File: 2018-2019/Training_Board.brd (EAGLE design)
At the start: 65 x 30 mm, 14 parts, among them IC1 ATMEGA328-20P, X1 JST-PH2

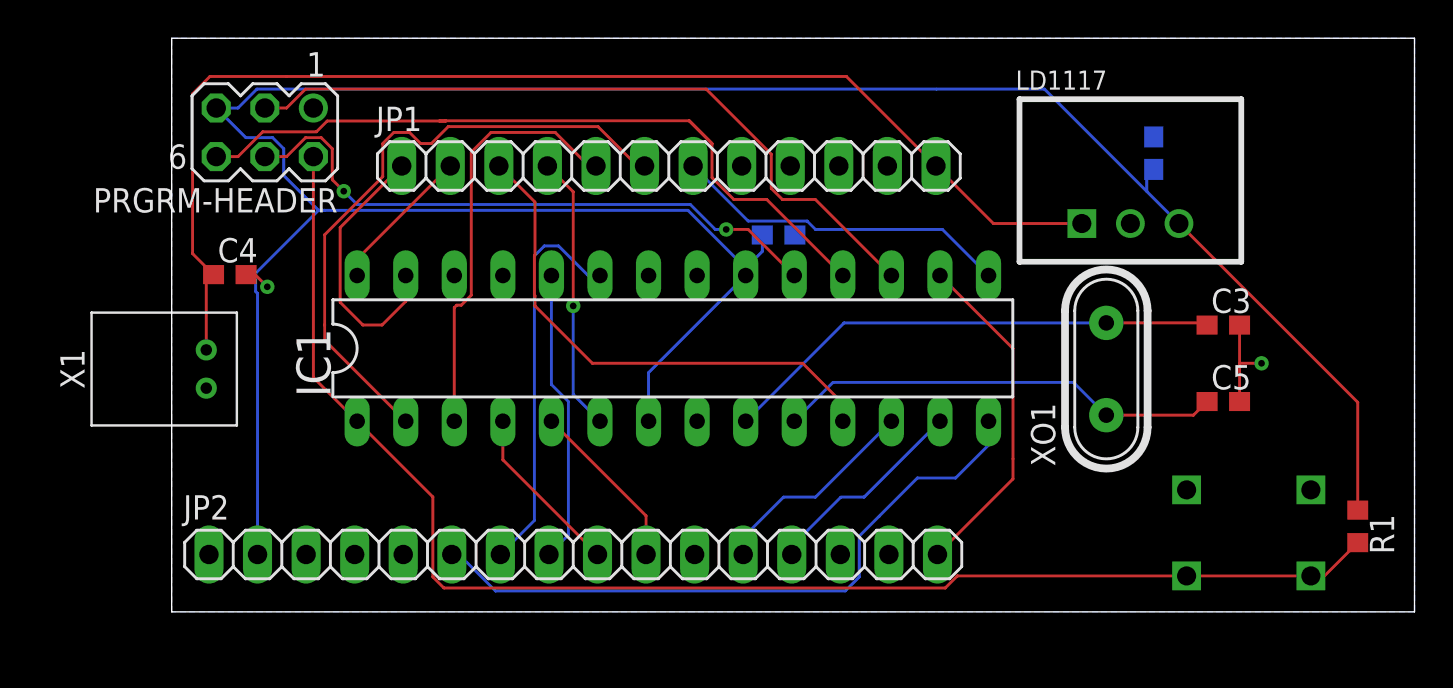
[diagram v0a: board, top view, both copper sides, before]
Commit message: Routed with larger trace widths and corrected pinouts
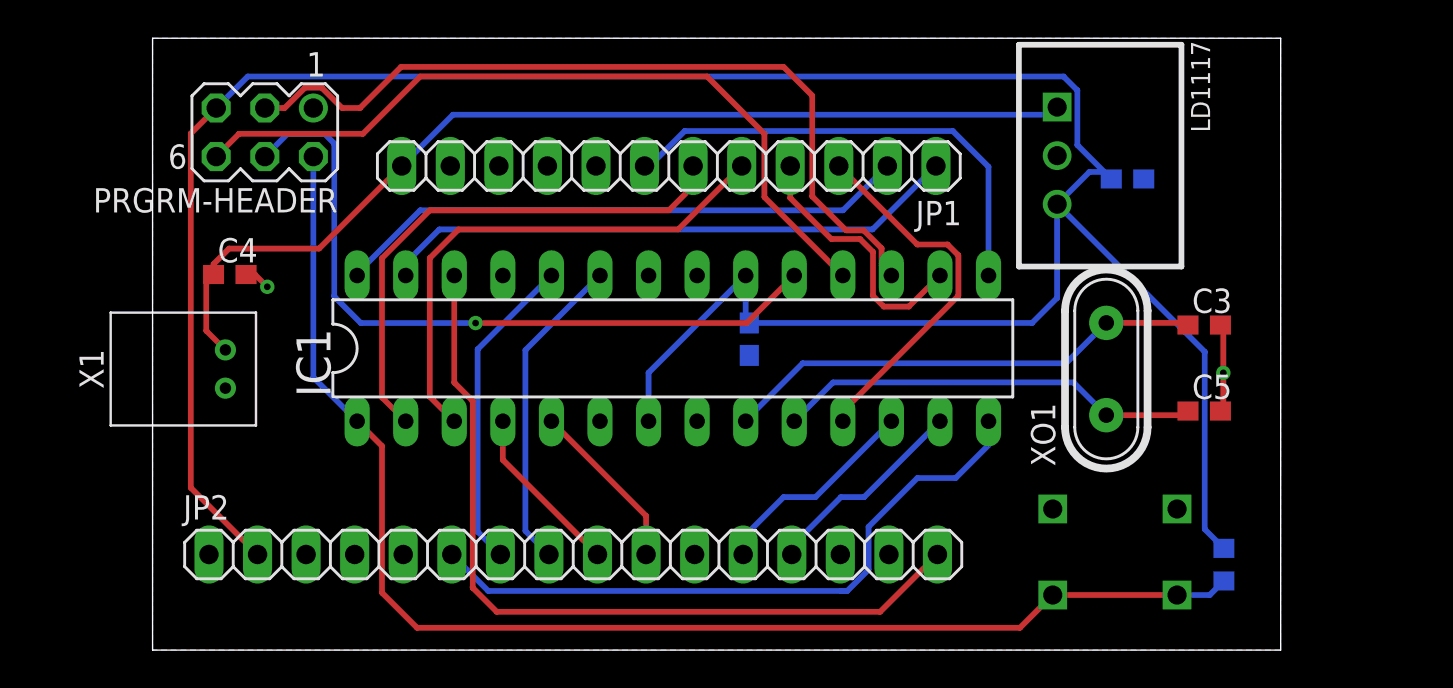
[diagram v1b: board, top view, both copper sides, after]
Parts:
- moved R1 7.28 mm to (55.0, 2.47), flipped to the bottom
- moved S1 7.07 mm to (46.1, 0.88)
- moved C1 5.66 mm to (30.2, 14.3), turned to 270 degrees
- moved LD1117 5.22 mm to (46.3, 23.9), turned to 270 degrees
- moved C2 1.92 mm to (50.0, 22.6), turned to 180 degrees
- moved C5 1.12 mm to (54.0, 10.5)
- moved C3 1.00 mm to (54.0, 15.0)
- moved X1 1.00 mm to (2.81, 12.7)
- turned JP1 to 180 degrees
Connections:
- net LIFT_A: now also IC1.16; no longer IC1.6
- net LINE_OUT_1: now also IC1.24; no longer IC1.23
- net LINE_OUT_2: now also IC1.23; no longer IC1.24
- net MOTOR_FAULT: now also IC1.26; no longer IC1.16
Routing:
- net MOTOR_FAULT: track 17.8 -> 42.8 mm
- net SCL: track 7.75 -> 30.2 mm
- net SDA: track 14.2 -> 30.5 mm
- net VBAT: track 64.1 -> 52.6 mm
- net LIFT_B: track 27.3 -> 19.4 mm
- net LEFT_B: track 17.8 -> 25.2 mm
- net SCK: track 32.0 -> 38.0 mm, vias 2 -> 1
- net RIGHT_B: track 22.3 -> 27.4 mm
- net RIGHT_A: track 32.9 -> 27.9 mm
- net MOSI: track 38.3 -> 42.7 mm
- net RST: track 74.2 -> 70.1 mm
- net LINE_OUT_1: track 20.6 -> 16.7 mm
- net +3V3: track 137.4 -> 135.3 mm
- net LINE_OUT_2: track 15.4 -> 16.7 mm
- net N$4: track 23.4 -> 22.2 mm
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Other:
- board size 65 x 30 mm -> 59 x 32 mm

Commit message: Replaced Thru-Hole with SMD Button
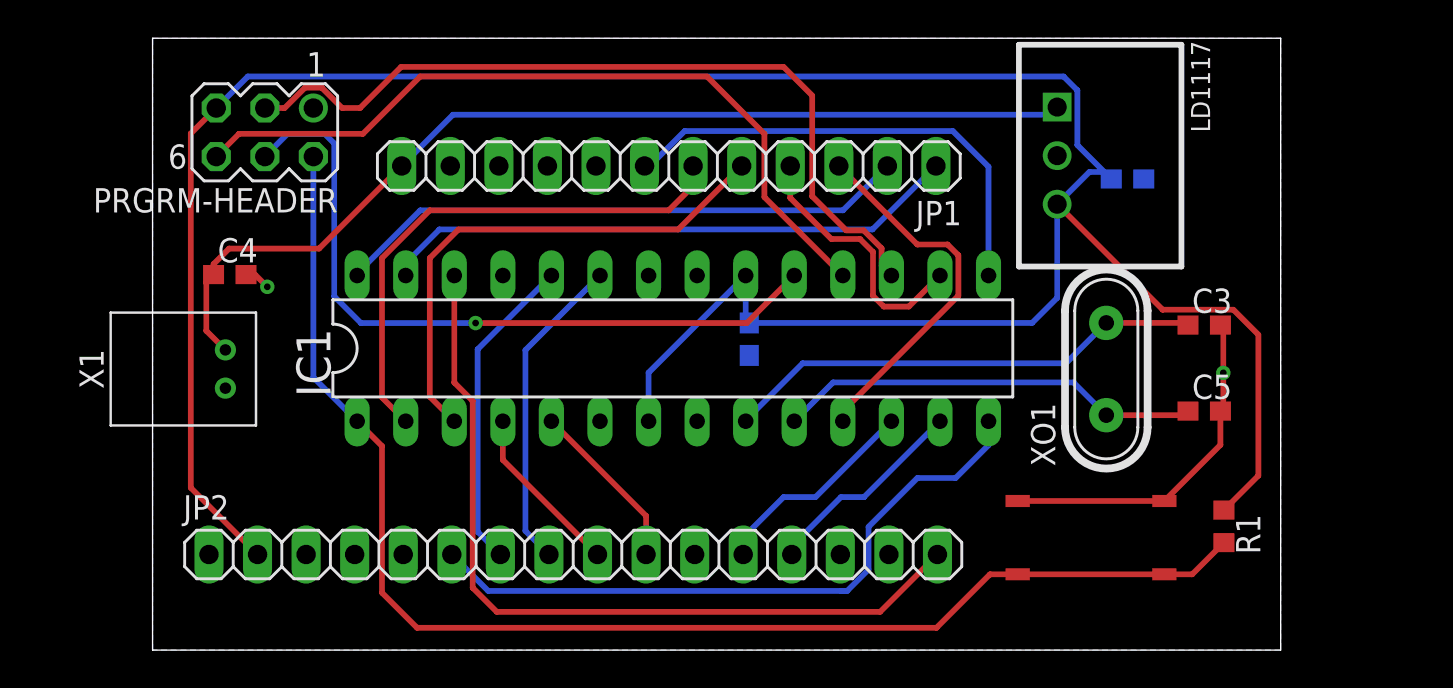
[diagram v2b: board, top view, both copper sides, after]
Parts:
- S1: value PTS645 -> PTS645PTS645_SMD1; device RoboJackets-Switches:PTS645 -> RoboJackets-Switches:PTS645_SMD
- moved S1 3.61 mm to (48.1, 3.88)
- moved R1 2.00 mm to (55.0, 4.47), flipped to the top
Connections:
- net GND: now also S1.P$1; no longer S1.P$3
- net RST: now also S1.P$3; no longer S1.P$1
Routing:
- net GND: track 6.00 -> 19.6 mm
- net +3V3: track 135.3 -> 137.0 mm
- net RST: track 70.1 -> 70.9 mm
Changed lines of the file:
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@@
 <attribute name="OC_NEWARK" value="unknown" x="4.87" y="25.08" size="1.778" layer="27" rot="R180" display="off"/>
 </element>
-<element name="R1" library="resistor" library_urn="urn:adsk.eagle:library:348" package="R0603" package3d_urn="urn:adsk.eagle:package:26057/1" value="10k Ohm" x="55.03" y="2.47" rot="MR270"/>
-<element name="S1" library="RoboJackets-Switches" package="PTS645" value="PTS645" x="46.08" y="0.88"/>
+<element name="R1" library="resistor" library_urn="urn:adsk.eagle:library:348" package="R0603" package3d_urn="urn:adsk.eagle:package:26057/1" value="10k Ohm" x="55.03" y="4.47" rot="R270"/>
+<element name="S1" library="RoboJackets-Switches" package="PTS645_SMD" value="PTS645PTS645_SMD1" x="48.08" y="3.88"/>
 <element name="X1" library="Trainii" package="JST-PH" value="JST-PH2" x="2.81" y="12.7" rot="R90"/>
 <element name="XO1" library="IQD-Frequency-Products" library_urn="urn:adsk.eagle:library:90" package="HC49" package3d_urn="urn:adsk.eagle:package:3356/1" value="CRYSTALS-NOGND-HC49/4H" x="48.88" y="12.7" rot="R90"/>
@@
 <contactref element="C5" pad="2"/>
 <contactref element="S1" pad="P$2"/>
-<contactref element="S1" pad="P$3"/>
+<contactref element="S1" pad="P$1"/>
 <contactref element="LD1117" pad="2"/>
 <contactref element="C2" pad="2"/>
@@
 <wire x1="54.85" y1="10.5" x2="55" y2="10.65" width="0.3" layer="1"/>
 <wire x1="55" y1="10.65" x2="55" y2="12.5" width="0.3" layer="1"/>
+<wire x1="44.245" y1="5.797" x2="51.915" y2="5.797" width="0.3" layer="1"/>
+<wire x1="54.85" y1="10.5" x2="54.85" y2="8.732" width="0.3" layer="1"/>
+<wire x1="54.85" y1="8.732" x2="51.915" y2="5.797" width="0.3" layer="1"/>
 </signal>
 <signal name="VBAT">
@@
 <contactref element="IC1" pad="1"/>
 <contactref element="R1" pad="2"/>
-<contactref element="S1" pad="P$1"/>
+<contactref element="S1" pad="P$3"/>
 <contactref element="S1" pad="P$4"/>
 <wire x1="7.41" y1="23.81" x2="7.41" y2="12.26" width="0.3" layer="16"/>
@@
 <wire x1="11" y1="8.67" x2="11" y2="1" width="0.3" layer="1"/>
 <wire x1="11" y1="1" x2="12.834" y2="-0.834" width="0.3" layer="1"/>
-<wire x1="12.834" y1="-0.834" x2="44.366" y2="-0.834" width="0.3" layer="1"/>
-<wire x1="44.366" y1="-0.834" x2="46.08" y2="0.88" width="0.3" layer="1"/>
-<wire x1="52.58" y1="0.88" x2="46.08" y2="0.88" width="0.3" layer="1"/>
-<wire x1="52.58" y1="0.88" x2="54.29" y2="0.88" width="0.3" layer="16"/>
-<wire x1="54.29" y1="0.88" x2="55.03" y2="1.62" width="0.3" layer="16"/>
+<wire x1="12.834" y1="-0.834" x2="40" y2="-0.834" width="0.3" layer="1"/>
+<wire x1="55.03" y1="3.62" x2="53.373" y2="1.963" width="0.3" layer="1"/>
+<wire x1="53.373" y1="1.963" x2="51.915" y2="1.963" width="0.3" layer="1"/>
+<wire x1="51.915" y1="1.963" x2="44.245" y2="1.963" width="0.3" layer="1"/>
+<wire x1="44.245" y1="1.963" x2="42.797" y2="1.963" width="0.3" layer="1"/>
+<wire x1="42.797" y1="1.963" x2="40" y2="-0.834" width="0.3" layer="1"/>
 </signal>
 <signal name="MISO">
@@
 <wire x1="30.02" y1="15.3" x2="30.21" y2="15.11" width="0.3" layer="16"/>
 <wire x1="2.33" y1="26.35" x2="3.98" y2="28" width="0.3" layer="16"/>
-<wire x1="54.03" y1="13.6" x2="54.03" y2="4.32" width="0.3" layer="16"/>
-<wire x1="55.03" y1="3.32" x2="54.03" y2="4.32" width="0.3" layer="16"/>
 <wire x1="30.21" y1="15.11" x2="45" y2="15.11" width="0.3" layer="16"/>
 <wire x1="47.3664" y1="24.4136" x2="48.775" y2="23.005" width="0.3" layer="16"/>
@@
 <wire x1="46.31" y1="21.32" x2="46.31" y2="16.42" width="0.3" layer="16"/>
 <wire x1="46.31" y1="16.42" x2="45" y2="15.11" width="0.3" layer="16"/>
-<wire x1="54.03" y1="13.6" x2="46.31" y2="21.32" width="0.3" layer="16"/>
+<wire x1="55.03" y1="5.32" x2="56.834" y2="7.124" width="0.3" layer="1"/>
+<wire x1="51.8276" y1="15.8024" x2="46.31" y2="21.32" width="0.3" layer="1"/>
+<wire x1="55.52525625" y1="15.8024" x2="51.8276" y2="15.8024" width="0.3" layer="1"/>
+<wire x1="56.834" y1="14.49365625" x2="55.52525625" y2="15.8024" width="0.3" layer="1"/>
+<wire x1="56.834" y1="7.124" x2="56.834" y2="14.49365625" width="0.3" layer="1"/>
 </signal>
 </signals>
